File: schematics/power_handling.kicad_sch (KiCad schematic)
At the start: 52 parts, among them J2 usb_c, SW1 CHS-01TA, U1 TPS62130, U12 FSUSB42MUX, U2 MIC5365-1.8YC5-TR, U3 TPS62130, U4 MIC5365-0.9YC5-TR

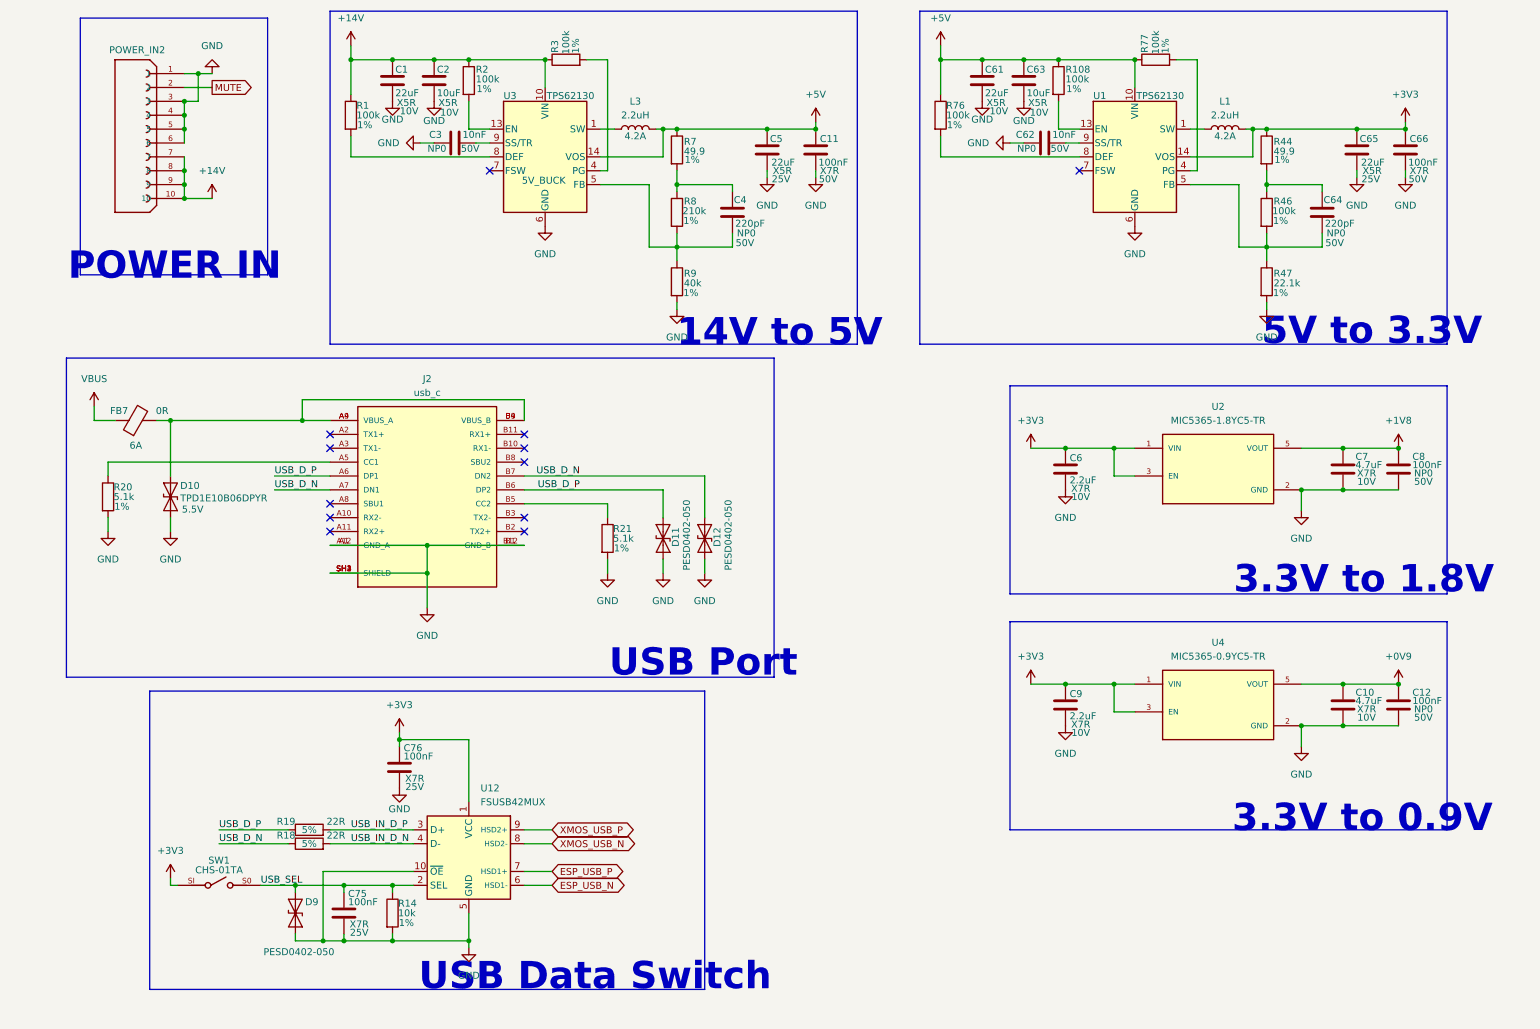
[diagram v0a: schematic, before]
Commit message: Add files via upload
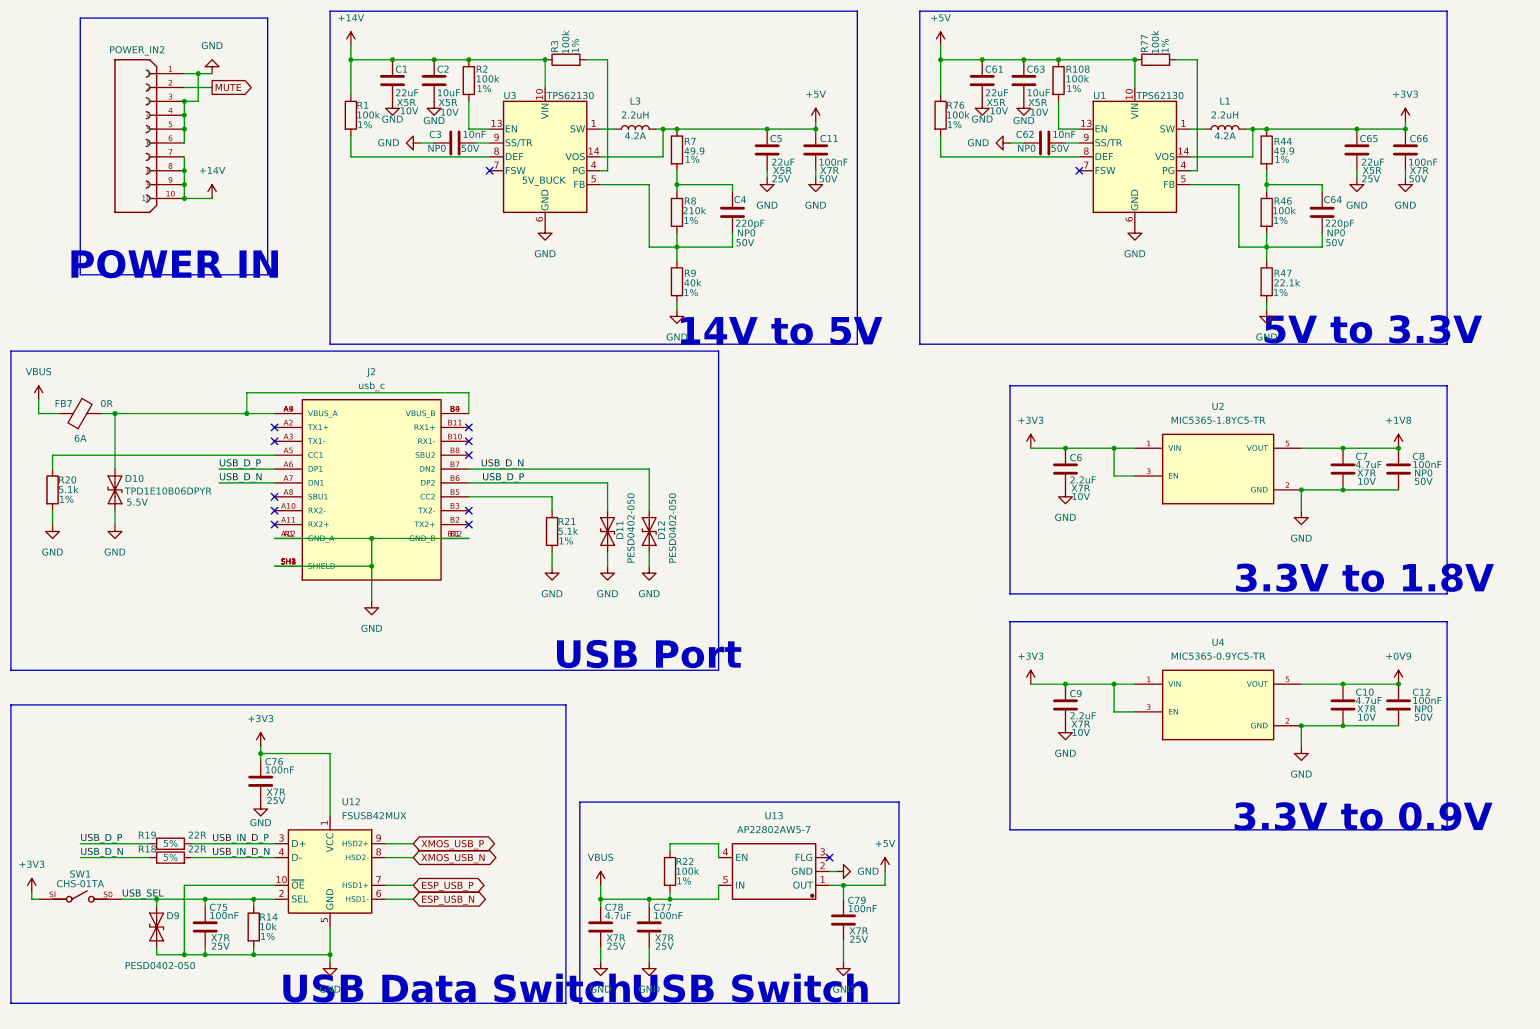
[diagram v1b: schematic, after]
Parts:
- added C77, C79: 100nF, Capacitor_SMD:C_0603_1608Metric, symbol Device:C
- added C78: 4.7uF, Capacitor_SMD:C_0603_1608Metric, symbol Device:C
- added R22: 100k, Resistor_SMD:R_0402_1005Metric, symbol Device:R
- added U13: AP22802AW5-7, Package_TO_SOT_SMD:SOT-23-5, symbol New_Library:AP22802AW5-7
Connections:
- net +5V: now also C79.1, U13.1 (OUT)
- net GND: now also C77.2, C78.2, C79.2, U13.2 (GND)
- net VBUS: now also C77.1, C78.1, R22.2, U13.5 (IN)
- new net: R22.1, U13.4 (EN)
- no-connect marks 12 -> 13
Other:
- note added: "USB Switch"
- moved on the sheet: C75, C76, D10, D11, D12, D9, FB7, J2, R14, R18, R19, R20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
